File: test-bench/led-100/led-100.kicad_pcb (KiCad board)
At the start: 2 copper layers, 17 parts, among them IC1 4511D, P1 CONN_02X05, U1 PC817, U2 PC817, U3 PC817, U4 PC817

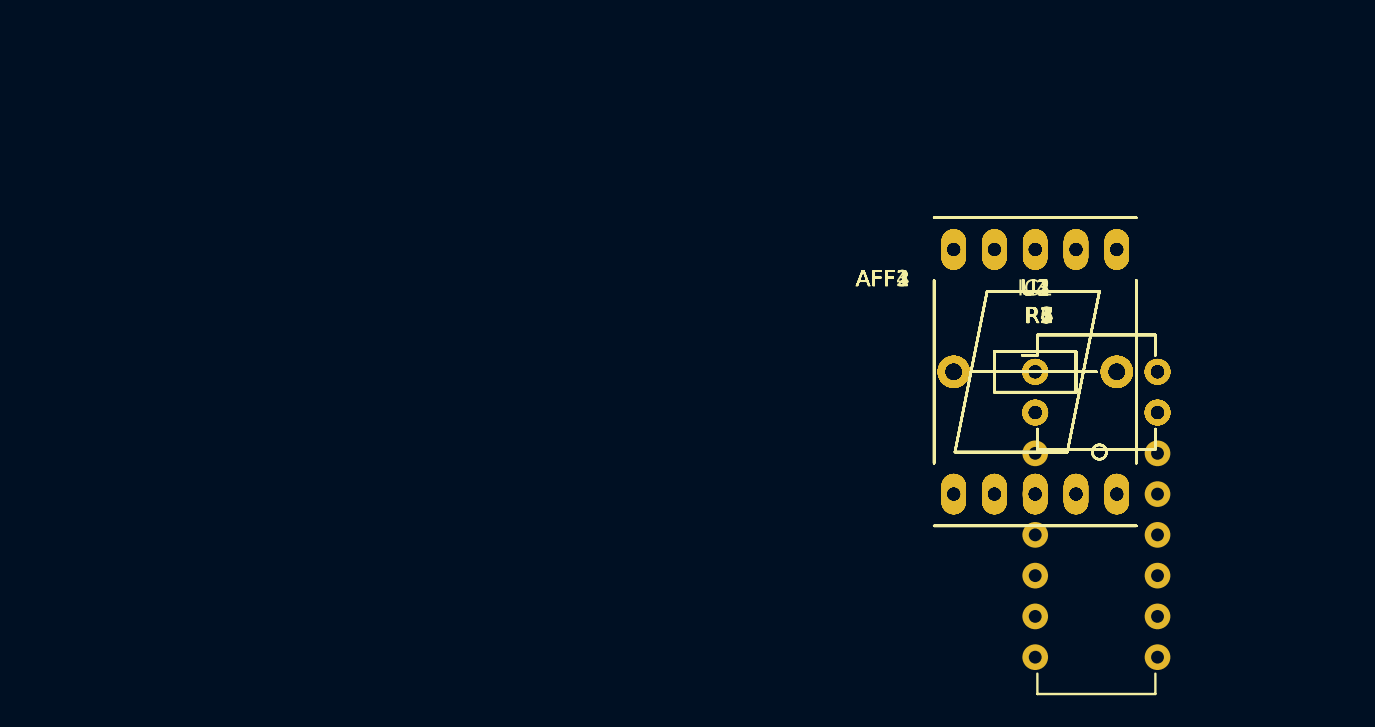
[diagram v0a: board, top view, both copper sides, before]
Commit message: BOM
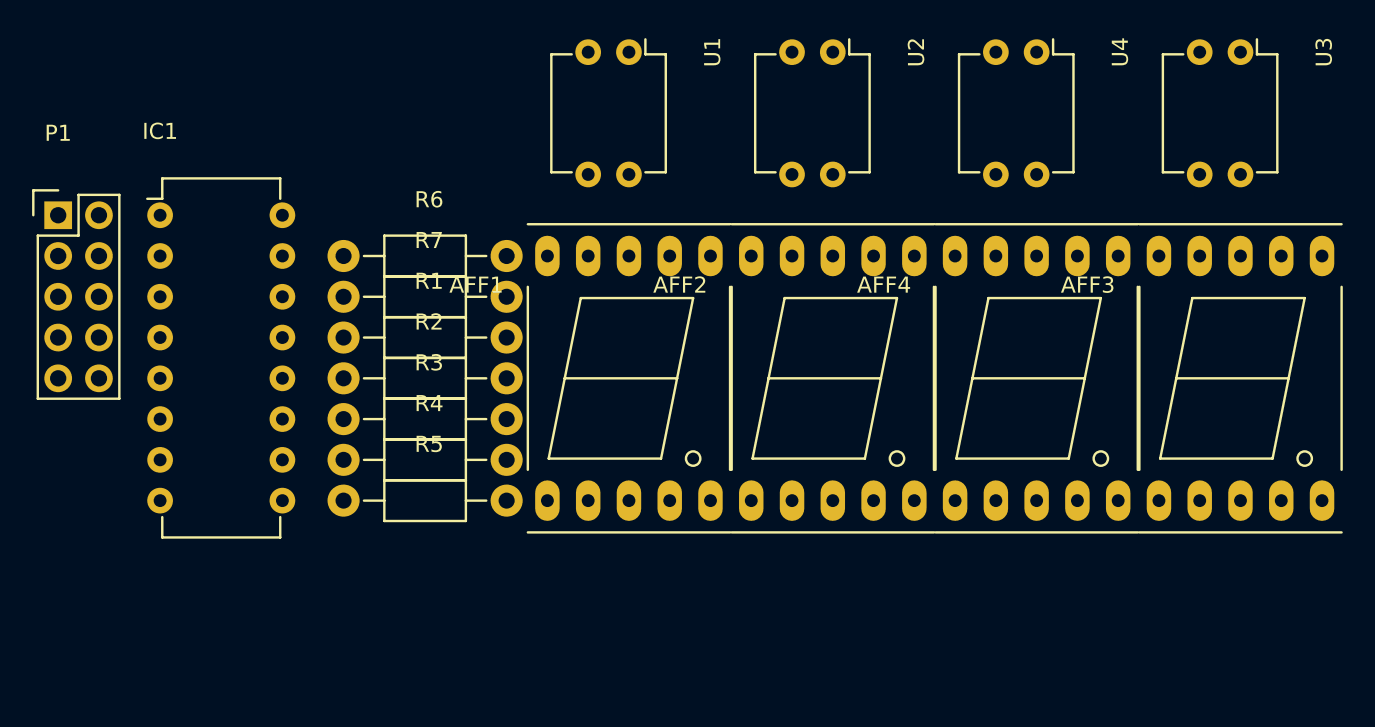
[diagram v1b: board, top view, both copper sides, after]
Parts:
- P1: footprint Resistors_ThroughHole:Resistor_Horizontal_RM10mm -> Pin_Headers:Pin_Header_Straight_2x05
- moved P1 61.6 mm to (87.6, 95.2)
- moved IC1 55.4 mm to (94.0, 95.2)
- moved R5 38.8 mm to (110.5, 113.0)
- moved R6 38.7 mm to (110.5, 97.8)
- moved R4 38.4 mm to (110.5, 110.5)
- moved R7 38.3 mm to (110.5, 100.3)
- moved R3 38.1 mm to (110.5, 108.0)
- moved R1 38.1 mm to (110.5, 102.9)
- moved R2 38.0 mm to (110.5, 105.4)
- moved U1 32.2 mm to (123.2, 85.1), turned to 270 degrees
- moved AFF1 25.3 mm to (123.2, 105.4)
- moved U3 23.7 mm to (161.3, 85.1), turned to 270 degrees
- moved U2 23.6 mm to (135.9, 85.1), turned to 270 degrees
- moved U4 19.9 mm to (148.6, 85.1), turned to 270 degrees
- moved AFF3 12.8 mm to (161.3, 105.4)
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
